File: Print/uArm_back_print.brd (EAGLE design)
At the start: 84 x 45 mm, 84 parts, among them IC1 ATmega644PA, IC2 ATTINY24/44/84-SSU, IC3 DCDC, IC4 DCDC, Q1 16MHz

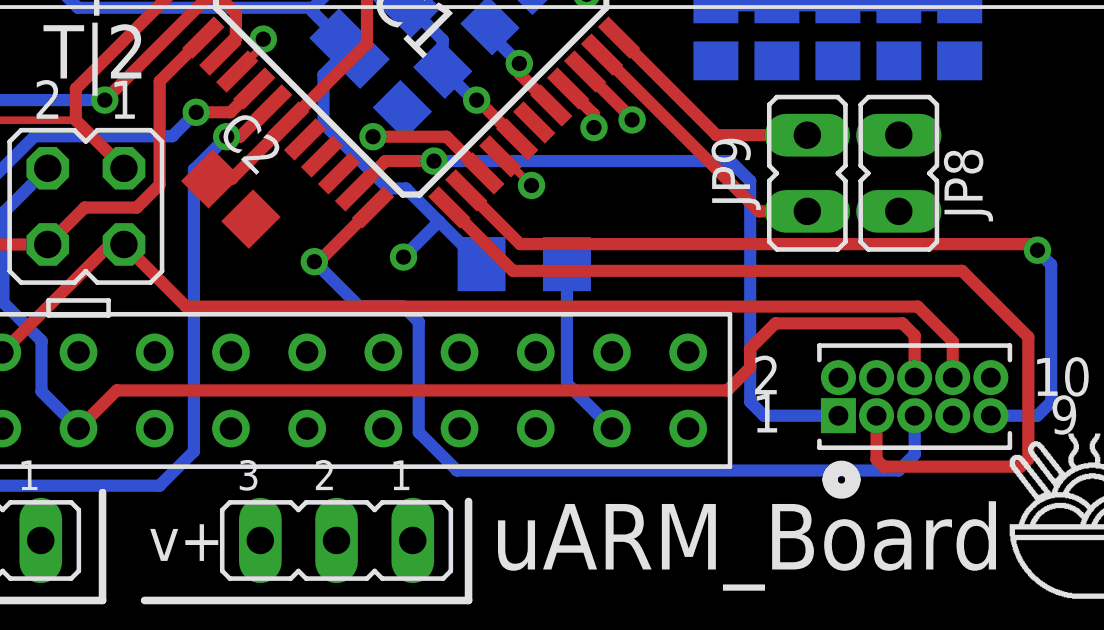
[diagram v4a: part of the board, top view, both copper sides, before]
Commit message: pijilj
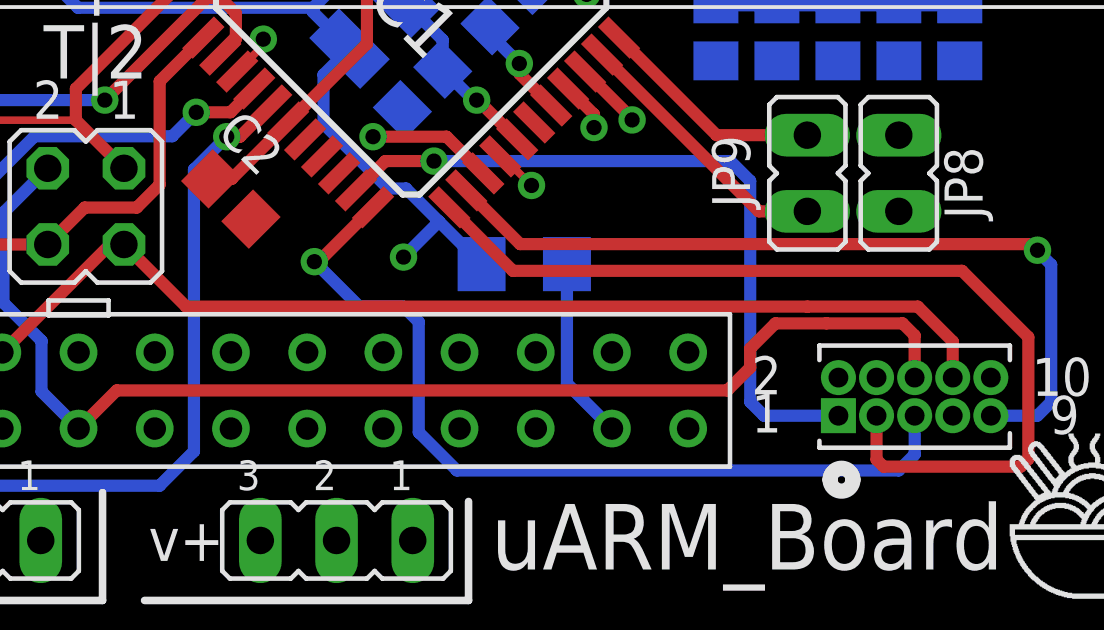
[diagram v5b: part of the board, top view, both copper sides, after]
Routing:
- net VCC: track 204.9 -> 205.5 mm
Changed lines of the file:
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@@
 <drawing>
 <settings>
-<setting alwaysvectorfont="yes"/>
+<setting alwaysvectorfont="no"/>
 <setting verticaltext="up"/>
 </settings>
@@
 <wire x1="51.6128" y1="19.559009375" x2="48.986759375" y2="16.93296875" width="0.4064" layer="1"/>
 <contactref element="LS" pad="C"/>
-<wire x1="68.6" y1="8.429" x2="68.2698" y2="8.7592" width="0.4064" layer="15"/>
-<wire x1="68.2698" y1="8.7592" x2="68.2698" y2="8.81828125" width="0.4064" layer="15"/>
-<wire x1="68.2698" y1="8.81828125" x2="66.29308125" y2="10.795" width="0.4064" layer="15"/>
-<wire x1="54.483" y1="10.795" x2="52.832" y2="12.446" width="0.4064" layer="15"/>
+<wire x1="52.832" y1="12.446" x2="54.483" y2="10.795" width="0.4064" layer="15"/>
 <via x="52.832" y="12.446" extent="1-16" drill="0.508"/>
 <wire x1="52.832" y1="12.446" x2="54.017" y2="13.631" width="0.4064" layer="16"/>
-<wire x1="66.29308125" y1="10.795" x2="54.483" y2="10.795" width="0.4064" layer="15"/>
 <wire x1="66.8811" y1="24.5682" x2="66.8811" y2="23.8281" width="0.4064" layer="16"/>
 <wire x1="66.8811" y1="23.8281" x2="66.421" y2="23.368" width="0.4064" layer="16"/>
@@
 <wire x1="57.754884375" y1="24.569721875" x2="58.9661625" y2="25.781" width="0.4064" layer="1"/>
 <wire x1="57.754884375" y1="24.569721875" x2="55.7403625" y2="22.5552" width="0.4064" layer="1"/>
+<wire x1="68.6" y1="9.632" x2="68.6" y2="8.429" width="0.4064" layer="15"/>
+<wire x1="54.483" y1="10.795" x2="67.437" y2="10.795" width="0.4064" layer="15"/>
+<wire x1="67.437" y1="10.795" x2="68.6" y2="9.632" width="0.4064" layer="15"/>
 </signal>
 <signal name="N$60">
@@
 <contactref element="U$4" pad="18"/>
 <wire x1="69.469" y1="10.2362" x2="69.87" y2="9.8352" width="0.4064" layer="1"/>
-<wire x1="69.469" y1="10.2362" x2="65.2272" y2="10.2362" width="0.4064" layer="1"/>
+<wire x1="69.469" y1="10.2362" x2="66.929" y2="10.2362" width="0.4064" layer="1"/>
+<wire x1="66.929" y1="10.2362" x2="65.2272" y2="10.2362" width="0.4064" layer="1"/>
 <wire x1="65.2272" y1="10.2362" x2="64.389" y2="9.398" width="0.4064" layer="1"/>
 <wire x1="64.389" y1="9.398" x2="64.389" y2="8.763" width="0.4064" layer="1"/>
@@
 <wire x1="43.514" y1="12.866" x2="45.585" y2="10.795" width="0.4064" layer="1"/>
 <wire x1="71.14" y1="9.632" x2="71.14" y2="8.429" width="0.4064" layer="1"/>
-<wire x1="45.585" y1="10.795" x2="69.977" y2="10.795" width="0.4064" layer="1"/>
+<wire x1="45.585" y1="10.795" x2="66.294" y2="10.795" width="0.4064" layer="1"/>
+<wire x1="66.294" y1="10.795" x2="69.977" y2="10.795" width="0.4064" layer="1"/>
 <wire x1="69.977" y1="10.795" x2="71.14" y2="9.632" width="0.4064" layer="1"/>
 </signal>
